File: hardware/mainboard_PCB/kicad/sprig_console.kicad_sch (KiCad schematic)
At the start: 25 parts, among them J1 1020_battery_holder, J2 Conn_PinHeader_2x03_P2.54mm_V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, SW1 W, SW2 A, SW3 S, SW4 D, SW5 I, SW6 J, SW7 K, SW8 L, SW9 Slideswitch, U1 Adafruit_TFT_ST7735, U2 MAX98357AETE+, U5 Pico

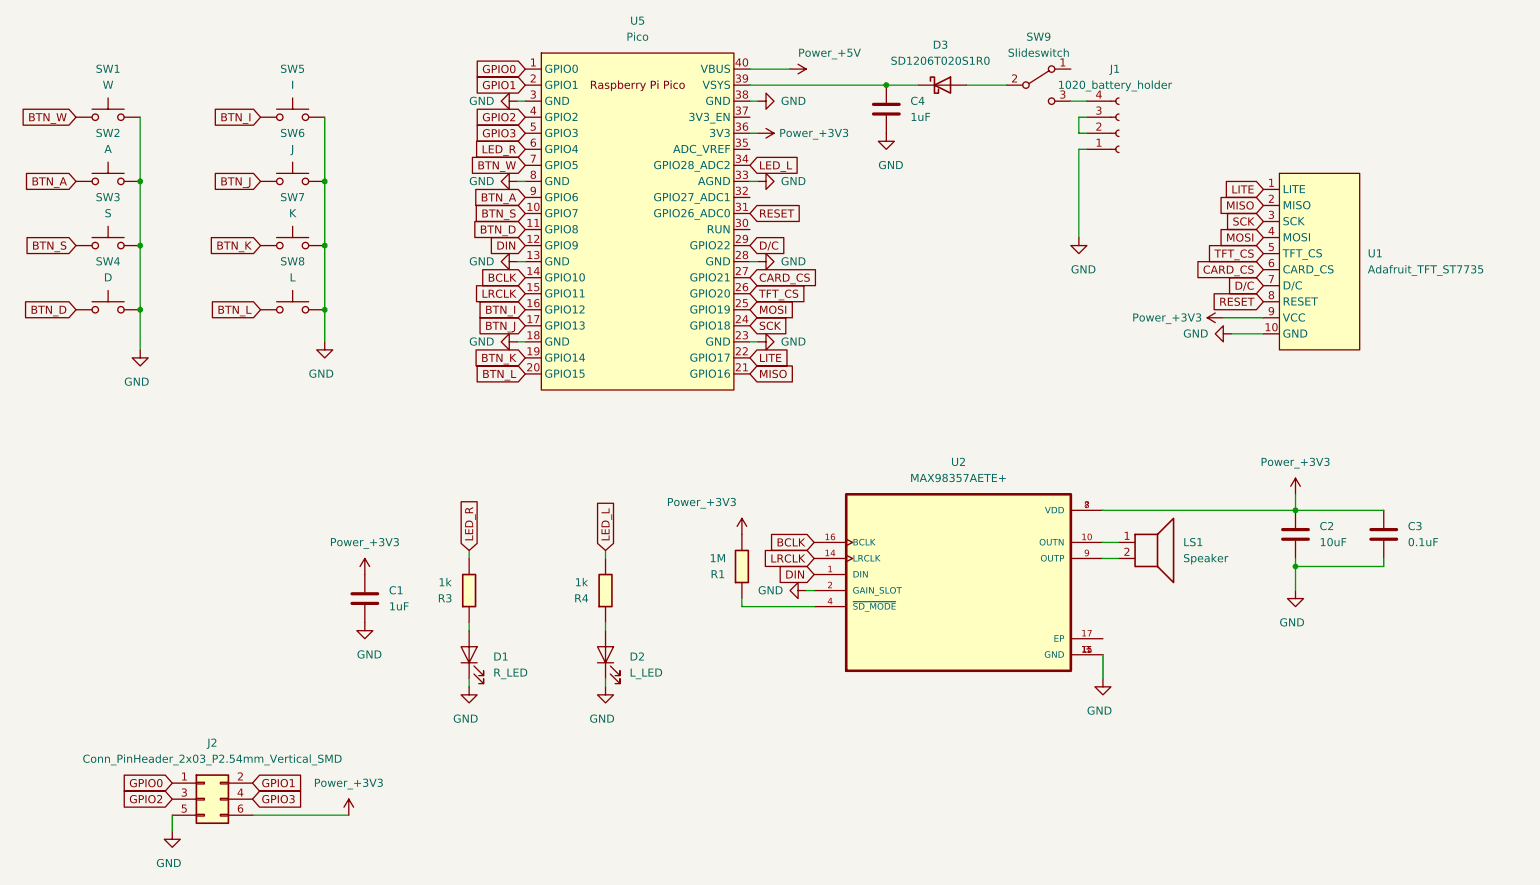
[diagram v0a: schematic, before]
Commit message: new board for new screen (#2430)
* new board design w/ cheaper screens

* new board design w/ cheaper screens

* add nora as co author

Co-authored-by: Nora <nora@hackclub.com>

* try again

wahoo



Co-authored-by: Nora <nora@hackclub.com>

* Update fp-lib-table


Co-authored-by: 24c02 <163450896+24c02@users.noreply.github.com>

---------

Co-authored-by: Nora <nora@hackclub.com>
Co-authored-by: 24c02 <163450896+24c02@users.noreply.github.com>
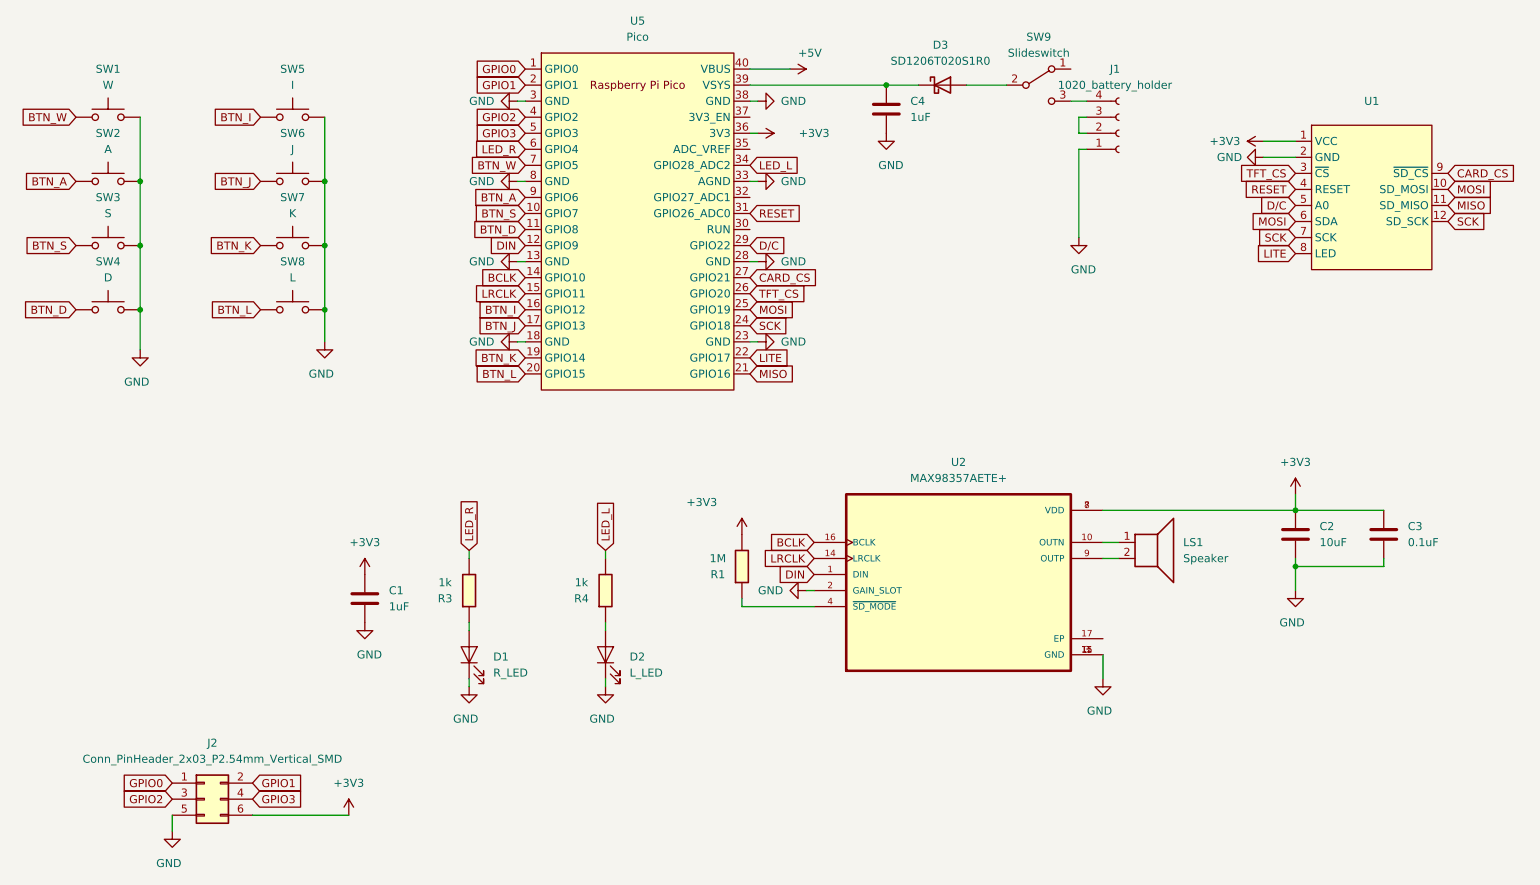
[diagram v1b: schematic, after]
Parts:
- removed U1: Adafruit_TFT_ST7735, fab:TFT_ST7735, symbol fab_custom:Adafruit_TFT_ST7735
- added U1: ~, sprig:TFT_MSP1803, symbol sprig:TFT_MSP1803
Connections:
- net +3V3: now also U1.1 (VCC)
- net CARD_CS: now also U1.9 (~{SD_CS})
- net D/C: now also U1.5 (A0)
- net GND: now also U1.2 (GND)
- net LITE: now also U1.8 (LED)
- net MISO: now also U1.11 (SD_MISO)
- net MOSI: now also U1.10 (SD_MOSI), U1.6 (SDA)
- net RESET: now also U1.4 (RESET)
- net SCK: now also U1.12 (SD_SCK), U1.7 (SCK)
- net TFT_CS: now also U1.3 (~{CS})
